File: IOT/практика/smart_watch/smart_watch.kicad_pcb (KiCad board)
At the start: 2 copper layers, 29 parts, among them J1 Conn_01x02_Pin, J2 USB_C_Receptacle_USB2.0_16P, SW3 SW_Push, U3 KXTJ3-1057, U4 MAX30102, U5 TPS61230DRC, U6 BQ24090DGQ, U7 ESP32-WROOM-32

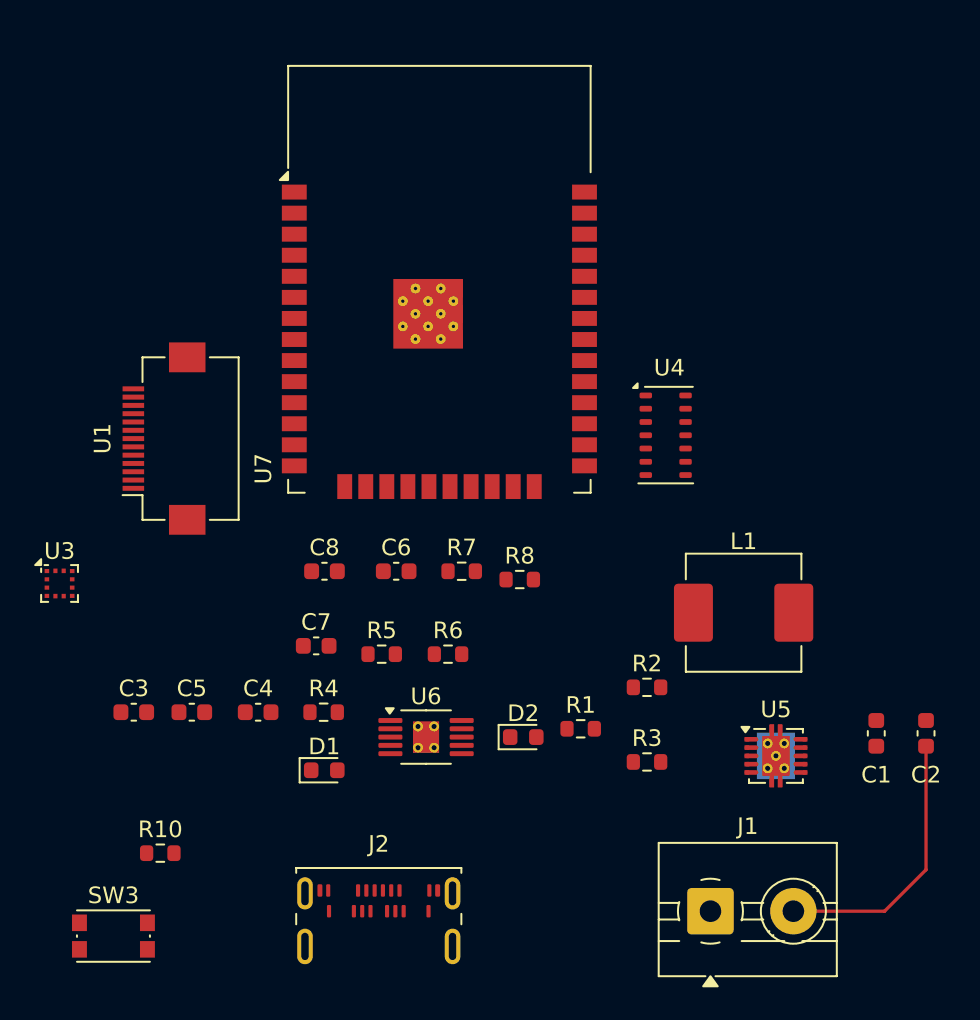
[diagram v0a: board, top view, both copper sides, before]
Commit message: updating smart watch
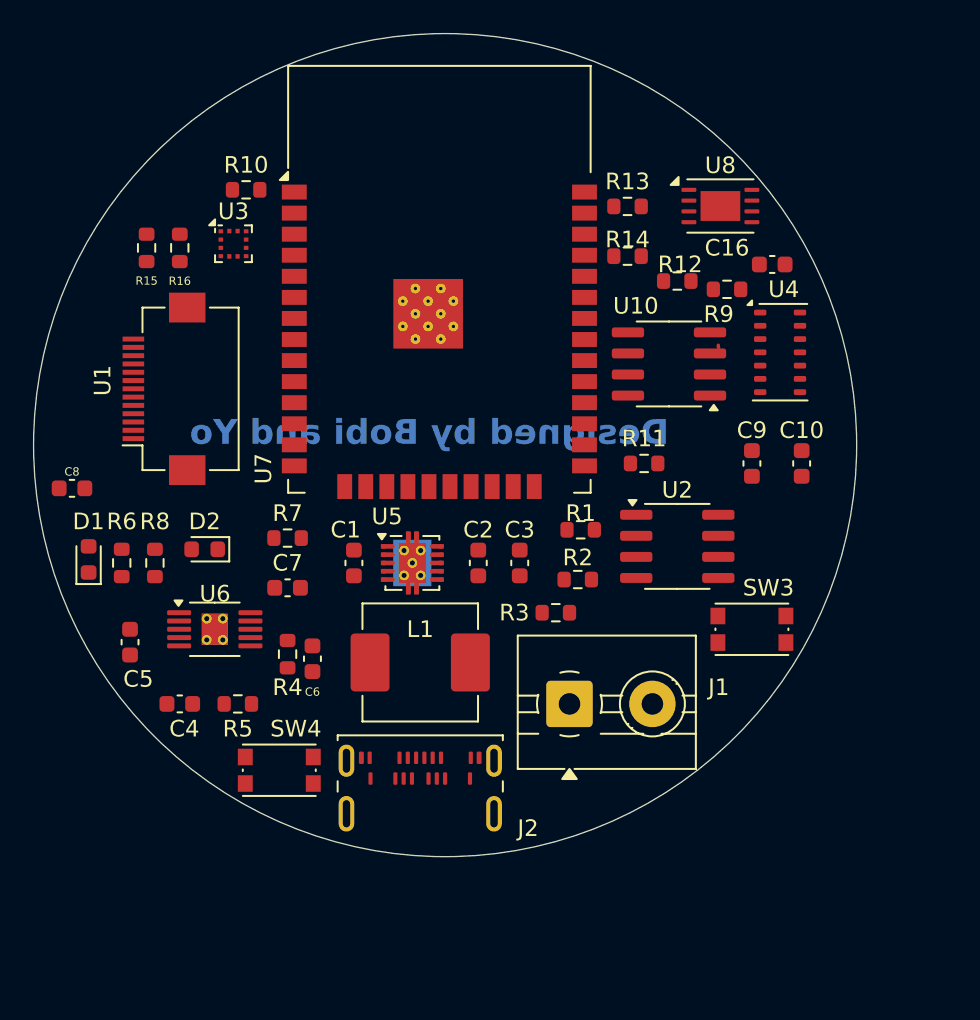
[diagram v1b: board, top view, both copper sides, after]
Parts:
- added C10: 0.1 uF, Capacitor_SMD:C_0603_1608Metric, F.Cu at (142.5, 107.0)
- added C16: 1uF, Capacitor_SMD:C_0603_1608Metric, F.Cu at (140.7, 95.0)
- added C9: 0.1 uF, Capacitor_SMD:C_0603_1608Metric, F.Cu at (139.5, 107.0)
- added R11: 10K, Resistor_SMD:R_0603_1608Metric, F.Cu at (133.0, 107.0)
- added R12: 10K, Resistor_SMD:R_0603_1608Metric, F.Cu at (135.0, 96.0)
- added R13: 10K, Resistor_SMD:R_0603_1608Metric, F.Cu at (132.0, 91.5)
- added R14: 10K, Resistor_SMD:R_0603_1608Metric, F.Cu at (132.0, 94.5)
- added R15: 10K, Resistor_SMD:R_0603_1608Metric, F.Cu at (103.0, 94.0)
- added R16: 10K, Resistor_SMD:R_0603_1608Metric, F.Cu at (105.0, 94.0)
- added R9: 10K, Resistor_SMD:R_0603_1608Metric, F.Cu at (138.0, 96.5)
- added SW4: SW_Push, Button_Switch_SMD:SW_Push_1P1T_NO_CK_KMR2, F.Cu at (111.0, 125.5)
- added U10: NLSV2T244D, Package_SO:SOIC-8_3.9x4.9mm_P1.27mm, F.Cu at (134.5, 101.0)
- added U2: CH330N, Package_SO:SOIC-8_3.9x4.9mm_P1.27mm, F.Cu at (135.0, 112.0)
- added U8: LC709203FQH-01TWG, Package_DFN_QFN:WDFN-8-1EP_4x3mm_P0.65mm_EP2.4x1.8mm, F.Cu at (137.6, 91.5)
- moved SW3 42.7 mm to (139.5, 117.0)
- moved R10 40.3 mm to (109.0, 90.5)
- moved C1 33.1 mm to (115.5, 113.0), turned to 90 degrees
- moved C2 28.9 mm to (123.0, 113.0), turned to 90 degrees
- moved C3 25.0 mm to (125.5, 113.0), turned to 90 degrees
- moved U5 24.8 mm to (119.0, 113.0)
- moved U3 23.0 mm to (108.2, 93.8)
- moved D2 22.3 mm to (106.5, 112.2), turned to 180 degrees
- moved R8 22.0 mm to (103.5, 113.0), turned to -90 degrees
- moved R6 20.4 mm to (101.5, 113.0), turned to -90 degrees
- moved L1 19.7 mm to (119.5, 119.0)
- moved D1 19.1 mm to (99.5, 112.8), turned to 90 degrees
- moved C8 16.0 mm to (98.5, 108.5)
- moved J1 15.1 mm to (128.5, 121.5)
- moved U6 14.3 mm to (107.1, 117.0)
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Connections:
- net Net-(U6-IN) renamed VBUS
- J2 pad A6: unconnected-(J2-D+-PadA6) -> D+
- J2 pad A7: unconnected-(J2-D--PadA7) -> D-
- R10 pad 1: Net-(U7-EN) -> +3V3
- R10 pad 2: GNDD -> Net-(U7-EN)
- SW3 pad 1: +3V3 -> GNDD
- U4 pad 11: 3V3 -> +3V3
- U7 pad 25: unconnected-(U7-IO0-Pad25) -> BOOT
- U7 pad 26: unconnected-(U7-IO4-Pad26) -> TP_RST
- U7 pad 27: TP_RST -> RX_2
- U7 pad 28: unconnected-(U7-IO17-Pad28) -> TX_2
- U7 pad 35: unconnected-(U7-TXD0/IO1-Pad35) -> TX
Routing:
- net GNDD: track 16.5 -> 0.00 mm
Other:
- board outline added: 49.6 x 49.6 mm
- board text added: "Designed by Bobi and Yo"
